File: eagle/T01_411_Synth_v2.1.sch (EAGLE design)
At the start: 25 parts, among them U1 ATMEGA328P, U2 74LVC1G08, U3 74LVC1G08

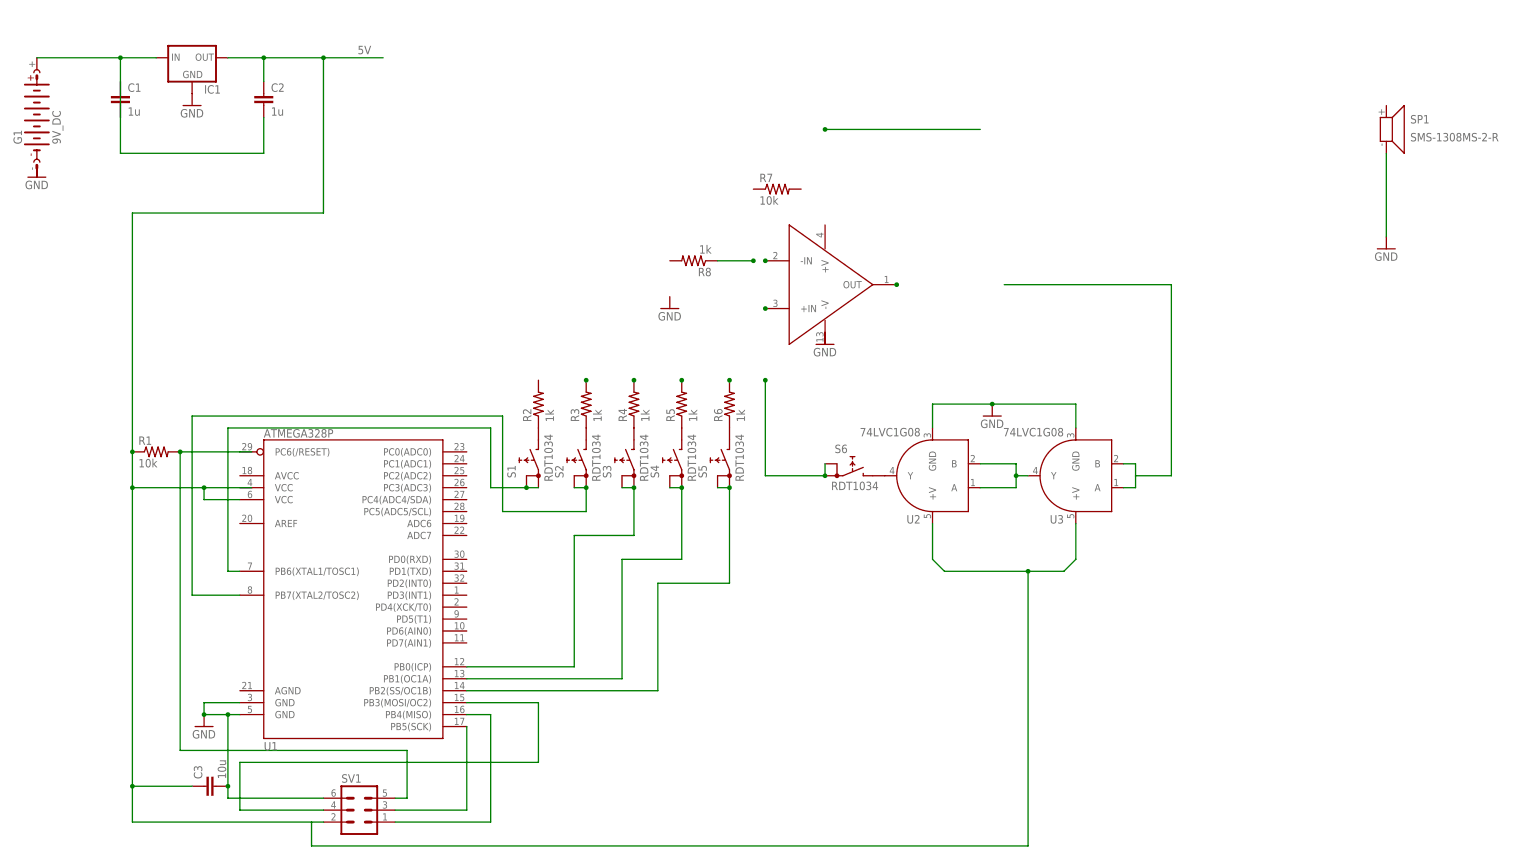
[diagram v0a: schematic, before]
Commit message: added libraries
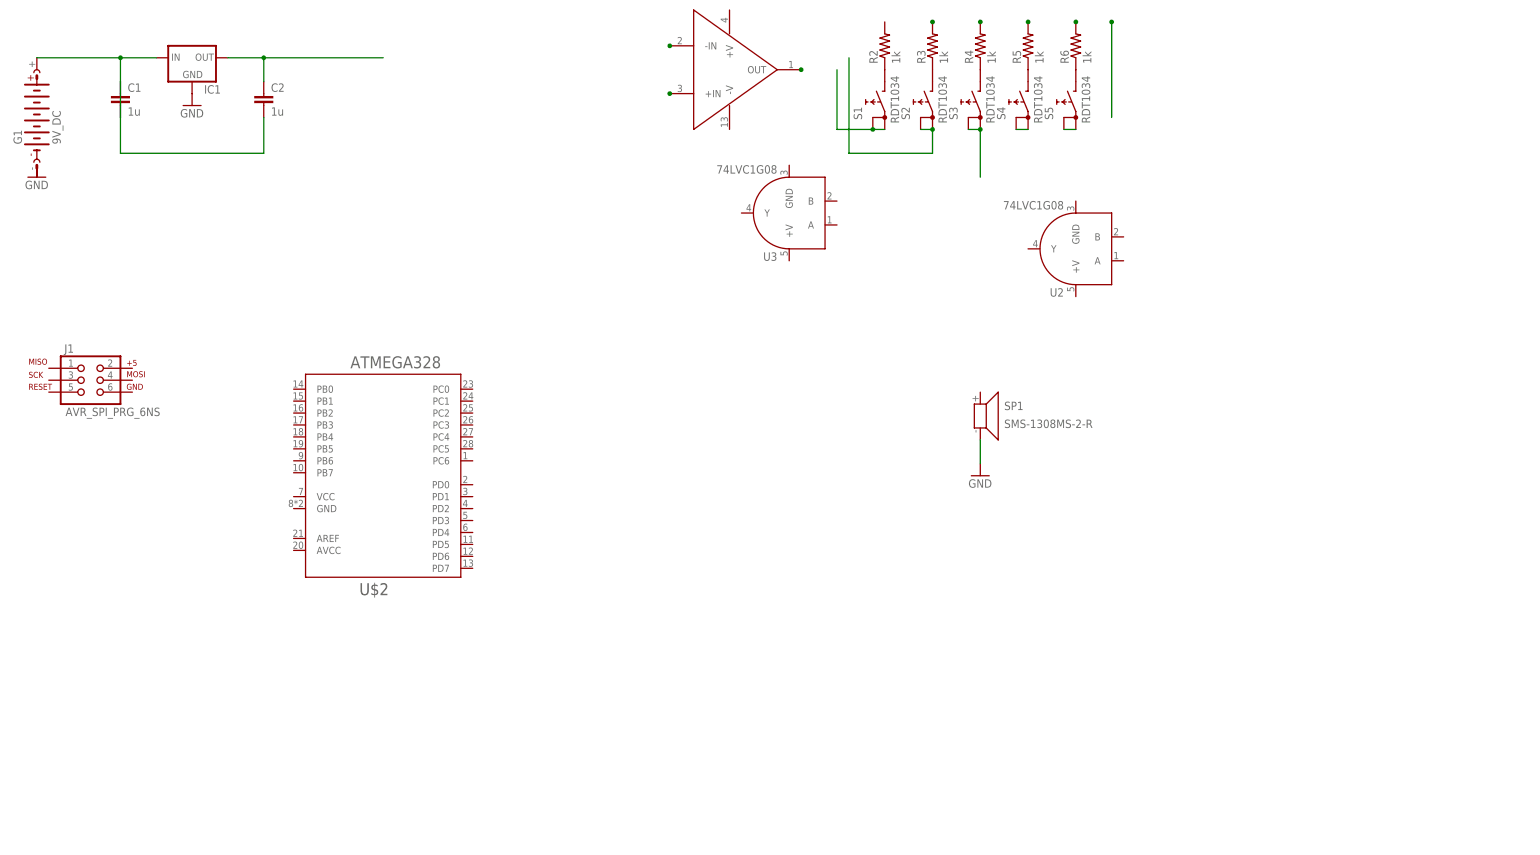
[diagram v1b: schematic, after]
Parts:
- removed C3: 10u, SparkFun-Capacitors:CAP0603-CAP
- removed R1, R7: 10k, SparkFun-Resistors:RESISTOR0603
- removed R8: 1k, SparkFun-Resistors:RESISTOR0603
- removed S6: RDT1034, switch:RDT1034
- removed SV1: (no value), con-lstb:MA03-2
- removed U1: ATMEGA328P, SparkFun-DigitalIC:ATMEGA328_SMT
- added J1: AVR_SPI_PRG_6NS, SparkFun-Connectors:AVR_SPI_PRG_6NS
- added U$2: ATMEGA328, libV2:ATMEGA328
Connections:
- removed net 5V: C2.1, C3.1, IC1.OUT, R1.1, SV1.2, U1.VCC@2, U2.+V, U3.+V
- removed net N$16: R8.1
- removed net N$2: SV1.4, U1.PB3(MOSI/OC2)
- removed net N$20: S6.A, S6.A1
- removed net N$3: SV1.1, U1.PB4(MISO)
- removed net N$5: R1.2, SV1.5, U1.PC6(/RESET)
- removed net N$6: S1.A, S1.A1, U1.PB6(XTAL1/TOSC1)
- removed net N$7: S2.A, S2.A1, U1.PB7(XTAL2/TOSC2)
- removed net N$9: S4.A, S4.A1, U1.PB1(OC1A)
- net GND: no longer C3.2, SV1.6, U1.GND@1, U2.GND, U3.GND
- net N$10: no longer U1.PB2(SS/OC1B)
- net N$19: now also S1.A, S1.A1; no longer S6.B, U2.Y
- net N$21: now also S2.A, S2.A1; no longer U2.A, U2.B, U3.Y
- net N$22: now also S4.A, S4.A1; no longer U3.A, U3.B
- net N$4: now also C2.1, IC1.OUT; no longer SV1.3, U1.PB5(SCK)
- net N$8: no longer U1.PB0(ICP)
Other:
- note removed: "A. Alavi"
- note removed: "Glove Synth"
- note removed: "J. Peirce"
- note removed: "N. Bryant"
- note removed: "N. Sayre"
- note removed: "Programmer"
- note removed: "T01"
- note removed: "delay reverb"
- note removed: "summing amp"
- moved on the sheet: R2, R3, R4, R5, R6, S1, S2, S3, S4, S5, SP1, U2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
